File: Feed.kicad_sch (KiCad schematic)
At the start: 38 parts

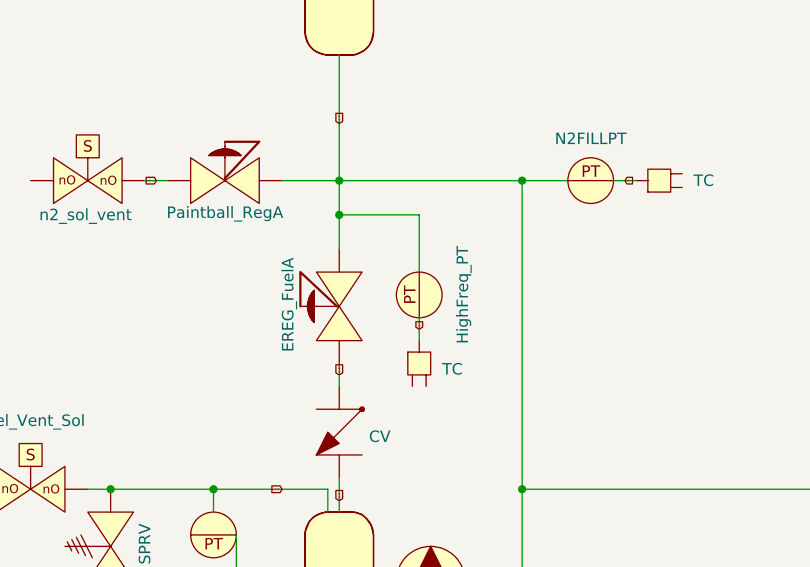
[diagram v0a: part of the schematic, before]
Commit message: PT Removal
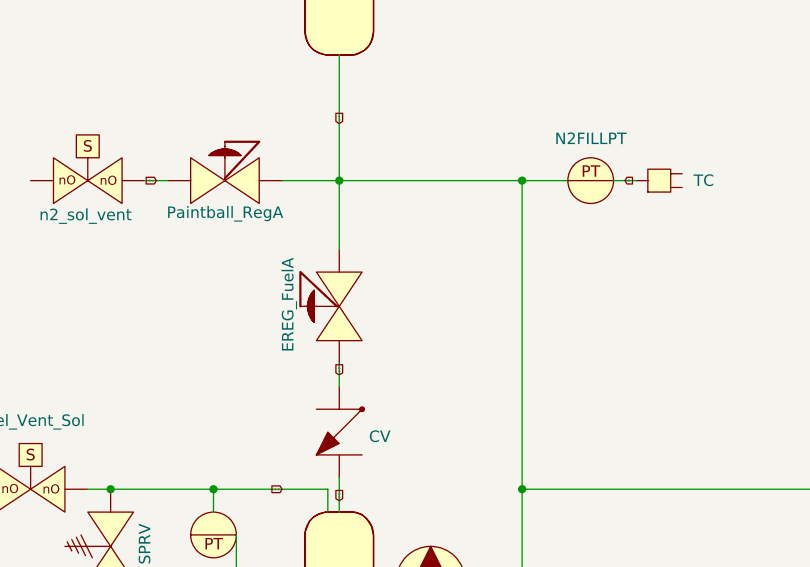
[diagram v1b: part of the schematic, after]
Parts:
- removed HighFreq_PT: ~, symbol PID_symbols:Pressure_Transducer
- removed TC: ~, symbol PID_symbols:Thermocouple
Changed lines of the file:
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@@
-	)
-	(junction
-		(at 106.68 88.9)
-		(diameter 0)
-		(color 0 0 0 0)
 	)
 	(junction
@@
 	(wire
 		(pts
-			(xy 106.68 85.09) (xy 106.68 88.9)
+			(xy 106.68 85.09) (xy 106.68 92.71)
 		)
 		(stroke
@@
 	(wire
 		(pts
-			(xy 115.57 88.9) (xy 106.68 88.9)
-		)
-		(stroke
-			(width 0)
-			(type default)
-		)
-	)
-	(wire
-		(pts
 			(xy 106.68 105.41) (xy 106.68 107.95)
 		)
@@
 	(wire
 		(pts
-			(xy 115.57 95.25) (xy 115.57 88.9)
-		)
-		(stroke
-			(width 0)
-			(type default)
-		)
-	)
-	(wire
-		(pts
 			(xy 106.68 165.1) (xy 120.65 165.1)
 		)
@@
 	(wire
 		(pts
-			(xy 115.57 100.33) (xy 115.57 102.87)
-		)
-		(stroke
-			(width 0)
-			(type default)
-		)
-	)
-	(wire
-		(pts
 			(xy 170.18 171.45) (xy 170.18 119.38)
 		)
@@
 		(pts
 			(xy 17.78 29.21) (xy 26.67 29.21)
-		)
-		(stroke
-			(width 0)
-			(type default)
-		)
-	)
-	(wire
-		(pts
-			(xy 106.68 88.9) (xy 106.68 92.71)
 		)
 		(stroke
@@
 				)
 				(justify right)
-				(hide yes)
-			)
-		)
-	)
-	(global_label "D"
-		(shape input)
-		(at 115.57 101.6 90)
-		(fields_autoplaced yes)
-		(effects
-			(font
-				(size 0.254 0.254)
-			)
-			(justify left)
-		)
-		(property "Intersheetrefs" "${INTERSHEET_REFS}"
-			(at 115.57 100.8794 90)
-			(effects
-				(font
-					(size 1.27 1.27)
-				)
-				(justify left)
 				(hide yes)
 			)
@@
 					(unit 1)
 				)
-			)
-		)
-	)
-	(symbol
-		(lib_name "Pressure_Transducer_1")
-		(lib_id "PID_symbols:Pressure_Transducer")
-		(at 115.57 97.79 90)
-		(unit 1)
-		(exclude_from_sim no)
-		(in_bom yes)
-		(on_board yes)
-		(dnp no)
-		(property "Reference" "HighFreq_PT"
-			(at 120.396 97.79 0)
-			(effects
-				(font
-					(size 1.27 1.27)
-				)
-			)
-		)
-		(property "Value" "~"
-			(at 116.84 97.79 0)
-			(effects
-				(font
-					(size 1.27 1.27)
-				)
-				(hide yes)
-			)
-		)
-		(property "Footprint" ""
-			(at 115.57 97.79 0)
-			(effects
-				(font
-					(size 1.27 1.27)
-				)
-				(hide yes)
-			)
-		)
-		(property "Datasheet" ""
-			(at 115.57 97.79 0)
-			(effects
-				(font
-					(size 1.27 1.27)
-				)
-				(hide yes)
-			)
-		)
-		(property "Description" ""
-			(at 115.57 97.79 0)
-			(effects
-				(font
-					(size 1.27 1.27)
-				)
-			)
-		)
-		(pin ""
-		)
-		(pin ""
-		)
-		(pin ""
-		)
-		(instances
-			(project "P_IDs"
-				(path "/045f1f05-3134-4b6d-91b6-463031104f1e/a0b6300e-76e9-4a18-afd6-e2d656b0d8f9/ac6f9866-6d7d-491d-94a4-140f8922d2b9"
-					(reference "HighFreq_PT")
-					(unit 1)
-				)
-			)
-		)
-	)
-	(symbol
-		(lib_id "PID_symbols:Thermocouple")
-		(at 115.57 105.41 0)
-		(unit 1)
-		(exclude_from_sim no)
-		(in_bom yes)
-		(on_board yes)
-		(dnp no)
-		(fields_autoplaced yes)
-		(property "Reference" "TC"
-			(at 118.11 106.0449 0)
-			(effects
-				(font
-					(size 1.27 1.27)
-				)
-				(justify left)
-			)
-		)
-		(property "Value" "~"
-			(at 115.57 105.41 0)
-			(effects
-				(font
-					(size 1.27 1.27)
-				)
-				(hide yes)
-			)
-		)
-		(property "Footprint" ""
-			(at 115.57 105.41 0)
-			(effects
-				(font
-					(size 1.27 1.27)
-				)
-				(hide yes)
-			)
-		)
-		(property "Datasheet" ""
-			(at 115.57 105.41 0)
-			(effects
-				(font
-					(size 1.27 1.27)
-				)
-				(hide yes)
-			)
-		)
-		(property "Description" ""
-			(at 115.57 105.41 0)
-			(effects
-				(font
-					(size 1.27 1.27)
-				)
-			)
-		)
-		(pin ""
-		)
-		(instances
-			(project "P_IDs"
-				(path "/045f1f05-3134-4b6d-91b6-463031104f1e/a0b6300e-76e9-4a18-afd6-e2d656b0d8f9/ac6f9866-6d7d-491d-94a4-140f8922d2b9"
-					(reference "TC")
-					(unit 1)
-				)
